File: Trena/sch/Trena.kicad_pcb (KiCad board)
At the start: 2 copper layers, 70.7 x 70.7 mm, 50 parts, among them J1 RJ45, J2 ICSP, J4 IN, J5 OUT, J6 HC-SR04, Q1 PN2222A, Q2 BC817-40, Q3 BC817-40, U1 ATMEGA328P-AU, U2 LM1117-5.0, U3 SP3485CN, Y1 Crystal

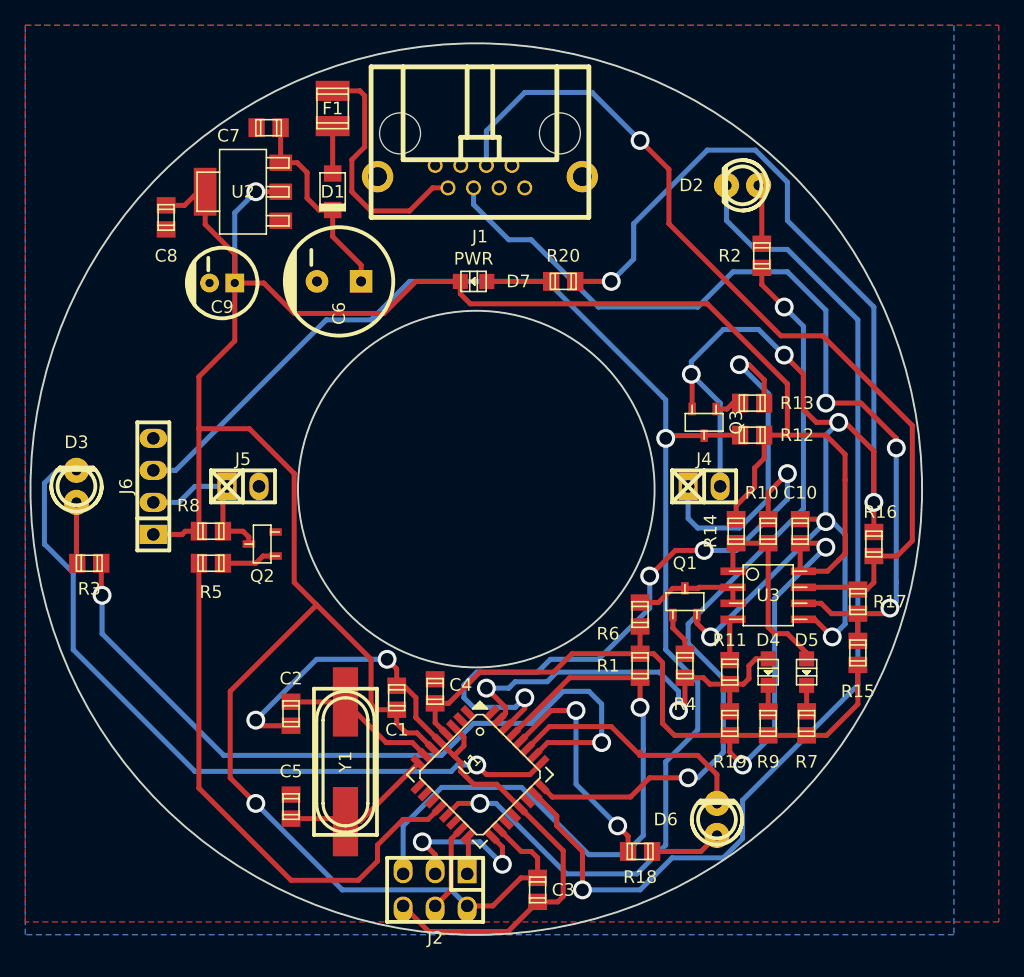
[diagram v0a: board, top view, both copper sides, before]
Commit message: Trena Posicionamento REV 3
Signed-off-by: cuki2 <mauricio@krebs.com.br>
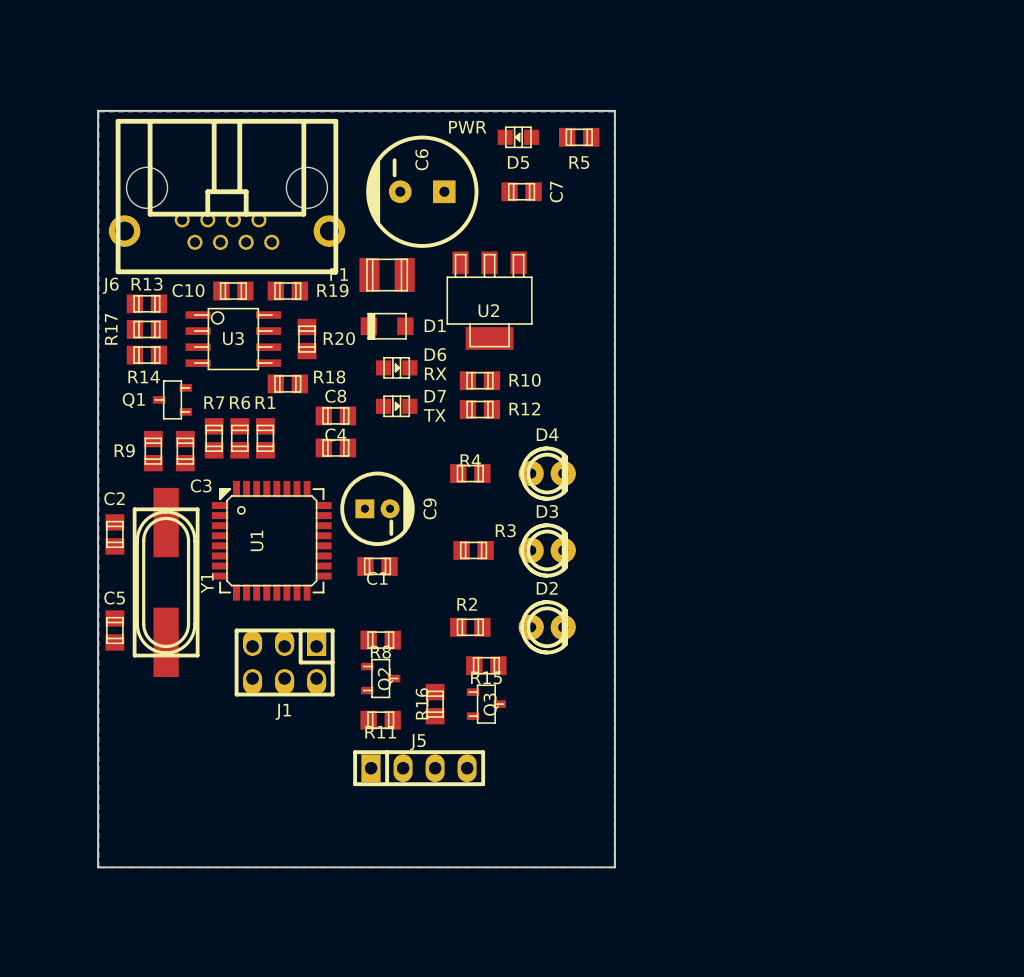
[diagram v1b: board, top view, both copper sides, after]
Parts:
- removed J2: ICSP, w_pin_strip:pin_strip_3x2
- removed J4: IN, w_pin_strip:pin_socket_2
- D4: value TX -> LED_3; footprint w_smd_leds:Led_0805 -> w_indicators:led_3mm_clear
- D5: value RX -> PWR
- D6: value LED_3 -> RX; footprint w_indicators:led_3mm_clear -> w_smd_leds:Led_0805
- D7: value PWR -> TX
- J1: value RJ45 -> ICSP; footprint w_conn_pc:rj45-shield -> w_pin_strip:pin_strip_3x2
- J5: value OUT -> HC-SR04; footprint w_pin_strip:pin_socket_2 -> w_pin_strip:pin_socket_4
- J6: value HC-SR04 -> RJ45; footprint w_pin_strip:pin_socket_4 -> w_conn_pc:rj45-shield
- R10: value 360R -> 560R
- R11: value 360R -> 10k
- R12, R19: value 10k -> 560R
- R13: value 1k -> 360R
- R14: value 10k -> 360R
- R15, R9: value 560R -> 10k
- R16, R7: value 560R -> 1k
- R17: value 120R -> 10k
- R18: value 120R -> 560R
- R20, R4: value 1k -> 120R
- R8: value 10k -> 1k
- moved R17 60.4 mm to (23.9, 37.3), turned to 180 degrees
- moved R9 53.3 mm to (24.4, 47.0)
- moved R7 52.1 mm to (29.2, 46.0), turned to 270 degrees
- moved R19 49.0 mm to (35.1, 34.3), turned to 180 degrees
- moved C10 48.8 mm to (30.7, 34.3), turned to 0 degrees
- moved R14 48.8 mm to (23.9, 39.4), turned to 0 degrees
- moved R13 48.6 mm to (23.9, 35.3), turned to 0 degrees
- moved D5 48.2 mm to (53.3, 22.1), turned to 180 degrees
- moved U3 47.0 mm to (30.7, 38.1)
- moved R18 46.4 mm to (35.1, 41.7)
- moved J1 44.7 mm to (34.8, 63.8)
- moved R5 44.7 mm to (58.2, 22.1)
- moved C3 44.6 mm to (26.9, 47.0), turned to 270 degrees
- moved D6 43.9 mm to (43.7, 40.4), turned to 0 degrees
- moved Q1 43.7 mm to (25.9, 42.9), turned to 90 degrees
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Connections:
- D4 pad 1: /TX -> Net-(D4-Pad1)
- D4 pad 2: Net-(D4-Pad2) -> /LED5
- D5 pad 2: Net-(D5-Pad2) -> +5V
- D6 pad 2: /LED5 -> Net-(D6-Pad2)
- D7 pad 1: Net-(D7-Pad1) -> /TX
- D7 pad 2: +5V -> Net-(D7-Pad2)
- J1 pad 1: GND -> /MISO
- J1 pad 2: /PIN -> +5V
- J1 pad 3: Net-(J1-Pad3) -> /SCK
- J1 pad 4: /A -> /MOSI
- J1 pad 5: /B -> /RESET
- J1 pad 6: Net-(J1-Pad6) -> GND
- J5 pad 1: Net-(J5-Pad1) -> +5V
- J5 pad 2: GND -> Net-(J4-Pad1)
- J6 pad 1: +5V -> GND
- J6 pad 2: Net-(J5-Pad1) -> /PIN
- J6 pad 3: /INT2 -> Net-(J6-Pad3)
- J6 pad 4: GND -> /A
- Q2 pad 2: Net-(J5-Pad1) -> Net-(J4-Pad1)
- R10 pad 1: Net-(D5-Pad1) -> Net-(D6-Pad2)
- R10 pad 2: /RX -> +5V
- R11 pad 1: Net-(R11-Pad1) -> +5V
- R11 pad 2: /TX -> Net-(J4-Pad1)
- R12 pad 2: /INT2 -> Net-(D7-Pad2)
- R13 pad 1: Net-(Q3-Pad1) -> Net-(D6-Pad1)
- R13 pad 2: Net-(J4-Pad1) -> /RX
- R14 pad 1: +5V -> Net-(R14-Pad1)
- R14 pad 2: Net-(D5-Pad1) -> /TX
- R15 pad 1: /A -> +5V
- R15 pad 2: +5V -> /INT2
- R16 pad 1: GND -> Net-(Q3-Pad1)
- R16 pad 2: /B -> Net-(J3-Pad1)
- R17 pad 1: /B -> +5V
- R17 pad 2: /A -> Net-(D6-Pad1)
- R18 pad 1: Net-(D6-Pad1) -> /A
- R18 pad 2: /LED6 -> +5V
- R19 pad 1: /TX -> GND
- R19 pad 2: +5V -> /B
- R20 pad 1: GND -> /B
- R20 pad 2: Net-(D7-Pad1) -> /A
- R4 pad 1: /TX -> Net-(D4-Pad1)
- R4 pad 2: Net-(Q1-Pad1) -> /LED6
- R5 pad 1: Net-(Q2-Pad1) -> GND
- R5 pad 2: /INT1 -> Net-(D5-Pad1)
- R6 pad 1: +5V -> /TX
- R6 pad 2: Net-(Q1-Pad2) -> +5V
- R7 pad 1: Net-(D5-Pad2) -> /TX
- R7 pad 2: +5V -> Net-(Q1-Pad1)
- R8 pad 1: +5V -> Net-(Q2-Pad1)
- R8 pad 2: Net-(J5-Pad1) -> /INT1
- R9 pad 2: Net-(D4-Pad2) -> Net-(Q1-Pad2)
- U3 pad 1: Net-(D5-Pad1) -> Net-(D6-Pad1)
- U3 pad 4: Net-(R11-Pad1) -> Net-(R14-Pad1)
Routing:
- net +5V: track 292.1 -> 0.00 mm, vias 4 -> 0
- net GND: track 191.9 -> 0.00 mm, vias 10 -> 0
- net /INT2: track 115.1 -> 0.00 mm, vias 2 -> 0
- net /LED1: track 85.0 -> 0.00 mm, vias 1 -> 0
- net /A: track 72.7 -> 0.00 mm, vias 3 -> 0
- net /B: track 71.9 -> 0.00 mm, vias 1 -> 0
- net /LED2: track 61.0 -> 0.00 mm, vias 2 -> 0
- net /LED4: track 60.6 -> 0.00 mm, vias 2 -> 0
- net /LED3: track 59.2 -> 0.00 mm, vias 1 -> 0
- net /RESET: track 51.5 -> 0.00 mm, vias 1 -> 0
- net /RX: track 49.0 -> 0.00 mm, vias 4 -> 0
- net /INT1: track 43.1 -> 0.00 mm
- net /TX: track 35.0 -> 0.00 mm, vias 2 -> 0
- net Net-(J4-Pad1): track 26.8 -> 0.00 mm, vias 1 -> 0
- net /LED5: track 20.2 -> 0.00 mm
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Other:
- board size 70.7 x 70.7 mm -> 41 x 60 mm
